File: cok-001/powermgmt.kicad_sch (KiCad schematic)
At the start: 29 parts, among them J6004 +12V_MAIN, J6005 +5V_EVER, Q6002 FDQ7238AS, U6003 MB39A, U6008 NCP511SN18T1, U6011 NCP511, U6012 MM3141, U6014 MM1591, U6019 NCP511SN18T1, U6021 MM1591, U6022 MM1593

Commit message: southbridge
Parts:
- U6008, U6019: footprint Package_SO:TSOP-5_1.65x3.05mm_P0.95mm -> Package_TO_SOT_SMD:SOT-23-5
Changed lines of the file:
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@@
 			)
 		)
-		(property "Footprint" "Package_SO:TSOP-5_1.65x3.05mm_P0.95mm"
+		(property "Footprint" "Package_TO_SOT_SMD:SOT-23-5"
 			(at 257.81 55.245 0)
 			(effects
@@
 			)
 		)
-		(property "Footprint" "Package_SO:TSOP-5_1.65x3.05mm_P0.95mm"
+		(property "Footprint" "Package_TO_SOT_SMD:SOT-23-5"
 			(at 257.81 83.185 0)
 			(effects

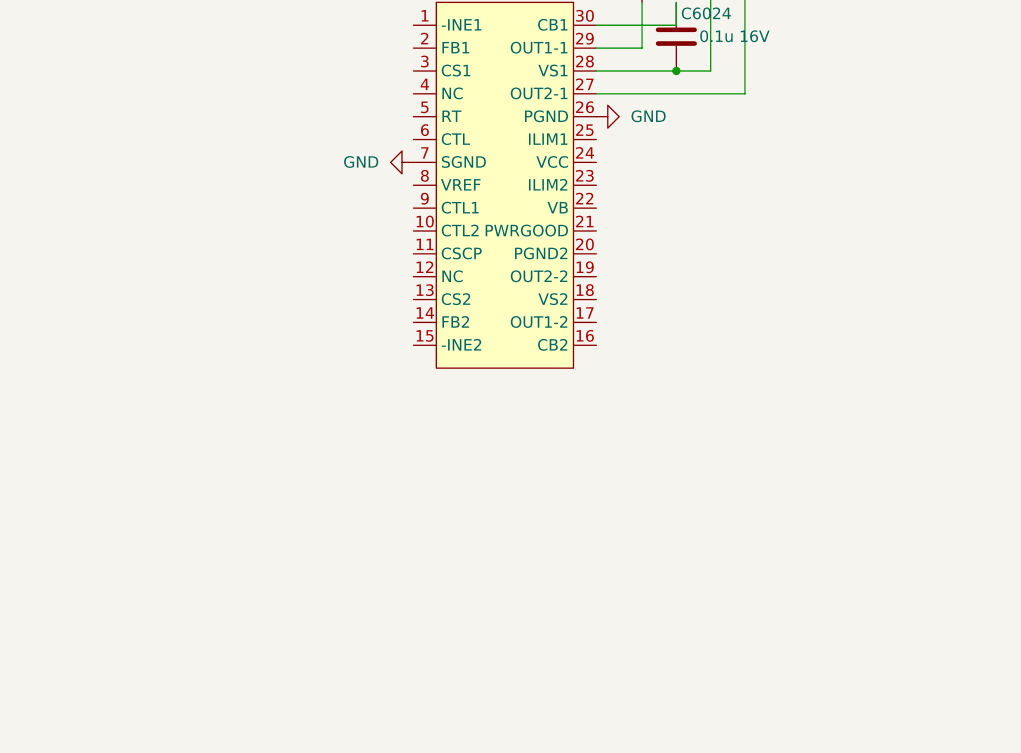
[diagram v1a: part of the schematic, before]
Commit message: sc
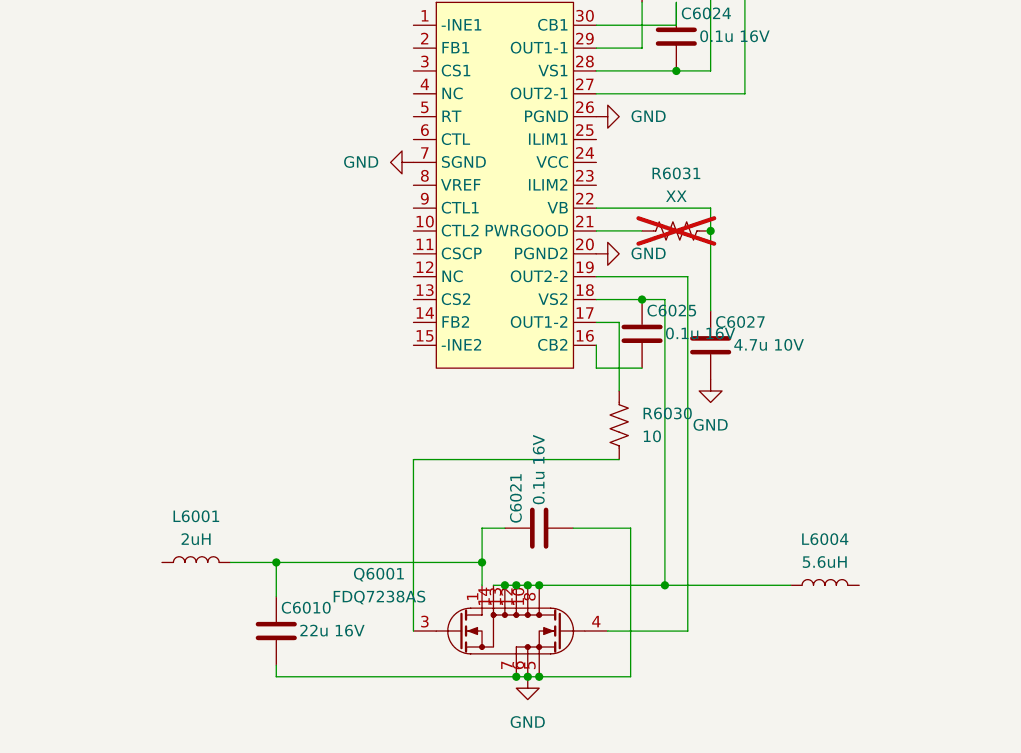
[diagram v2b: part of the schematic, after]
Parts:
- added C6010: 22u 16V, Capacitor_SMD:C_1210_3225Metric, symbol Device:C
- added C6021, C6025: 0.1u 16V, Capacitor_SMD:C_0603_1608Metric, symbol Device:C
- added C6027: 4.7u 10V, Capacitor_SMD:C_0805_2012Metric, symbol Device:C
- added L6001: 2uH, Inductor_SMD:L_TDK_SLF6028, symbol Device:L
- added L6004: 5.6uH, Inductor_SMD:L_TDK_SLF10145, symbol Device:L
- added Q6001: FDQ7238AS, Package_SO:SO-14_3.9x8.65mm_P1.27mm, symbol PS3:FDQ7238AS
- added R6030: 10, Resistor_SMD:R_0603_1608Metric, symbol Device:R_US
- added R6031: XX, Resistor_SMD:R_0402_1005Metric, symbol Device:R_US
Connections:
- net GND: now also U6003.20 (PGND2), C6010.2, C6021.2, C6027.2, Q6001.5 (D), Q6001.6, Q6001.7
- net at U6003.16 (CB2): now also C6025.2
- net at U6003.17 (OUT1-2): now also R6030.2
- net at U6003.18 (VS2): now also C6025.1, L6004.1, Q6001.10, Q6001.11, Q6001.12, Q6001.13, Q6001.14, Q6001.8, Q6001.9
- net at U6003.19 (OUT2-2): now also Q6001.4 (G)
- net at U6003.21 (PWRGOOD): now also R6031.2
- net at U6003.22 (VB): now also C6027.1, R6031.1
- new net: C6010.1, C6021.1, L6001.2, Q6001.1 (S), Q6001.2 (S)
- new net: Q6001.3 (S), R6030.1
